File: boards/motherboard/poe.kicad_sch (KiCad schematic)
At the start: 51 parts, among them Q1 FDC2512, T1 HR051067, U2 TPS23753APWR, U3 FOD817AS, U4 TLV341ASN1

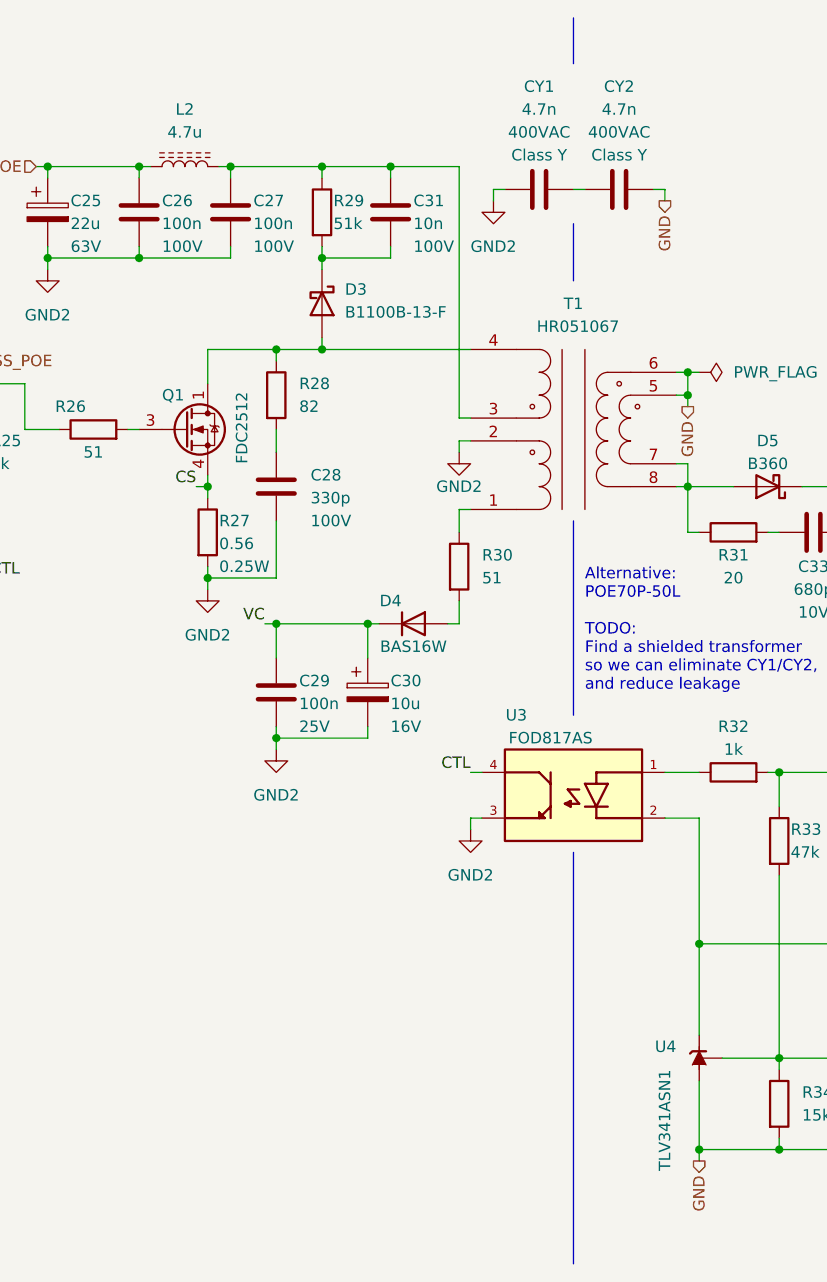
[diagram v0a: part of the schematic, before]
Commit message: feat: first revision of pcb layout
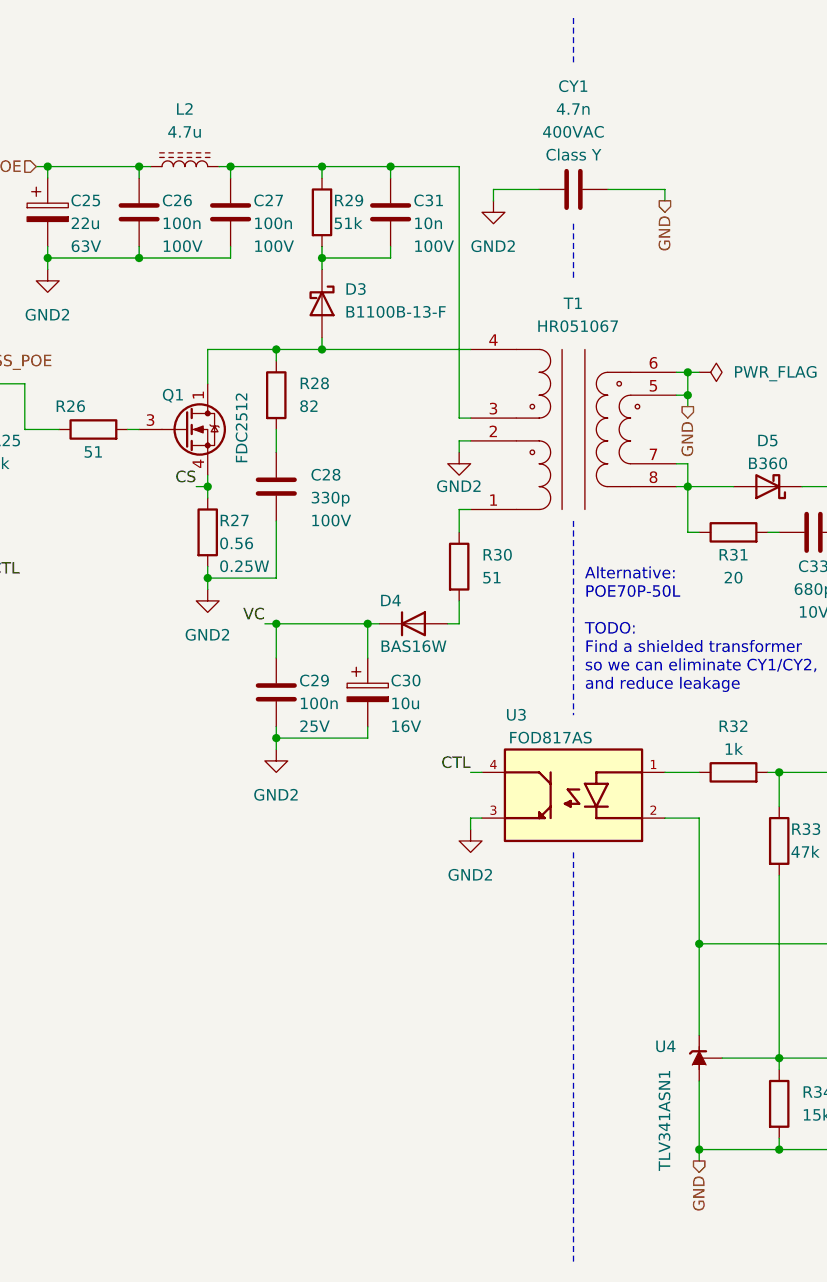
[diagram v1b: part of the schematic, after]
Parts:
- removed CY2: 4.7n, Capacitor_THT:C_Disc_D10.5mm_W5.0mm_P10.00mm, symbol Device:C
- T1: footprint footprints:XFMR-SMD_HR051067 -> HR051067:HR051067
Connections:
- net GND: now also CY1.1
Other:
- moved on the sheet: CY1
